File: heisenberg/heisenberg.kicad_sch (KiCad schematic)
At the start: 5 parts, among them J1 HLE-110-02-L-DV-BE-K-TR, J2 HLE-110-02-L-DV-BE-K-TR, J3 TSM-108-01-F-DV, J4 S16B-XH-A, U1 Teensy4.1

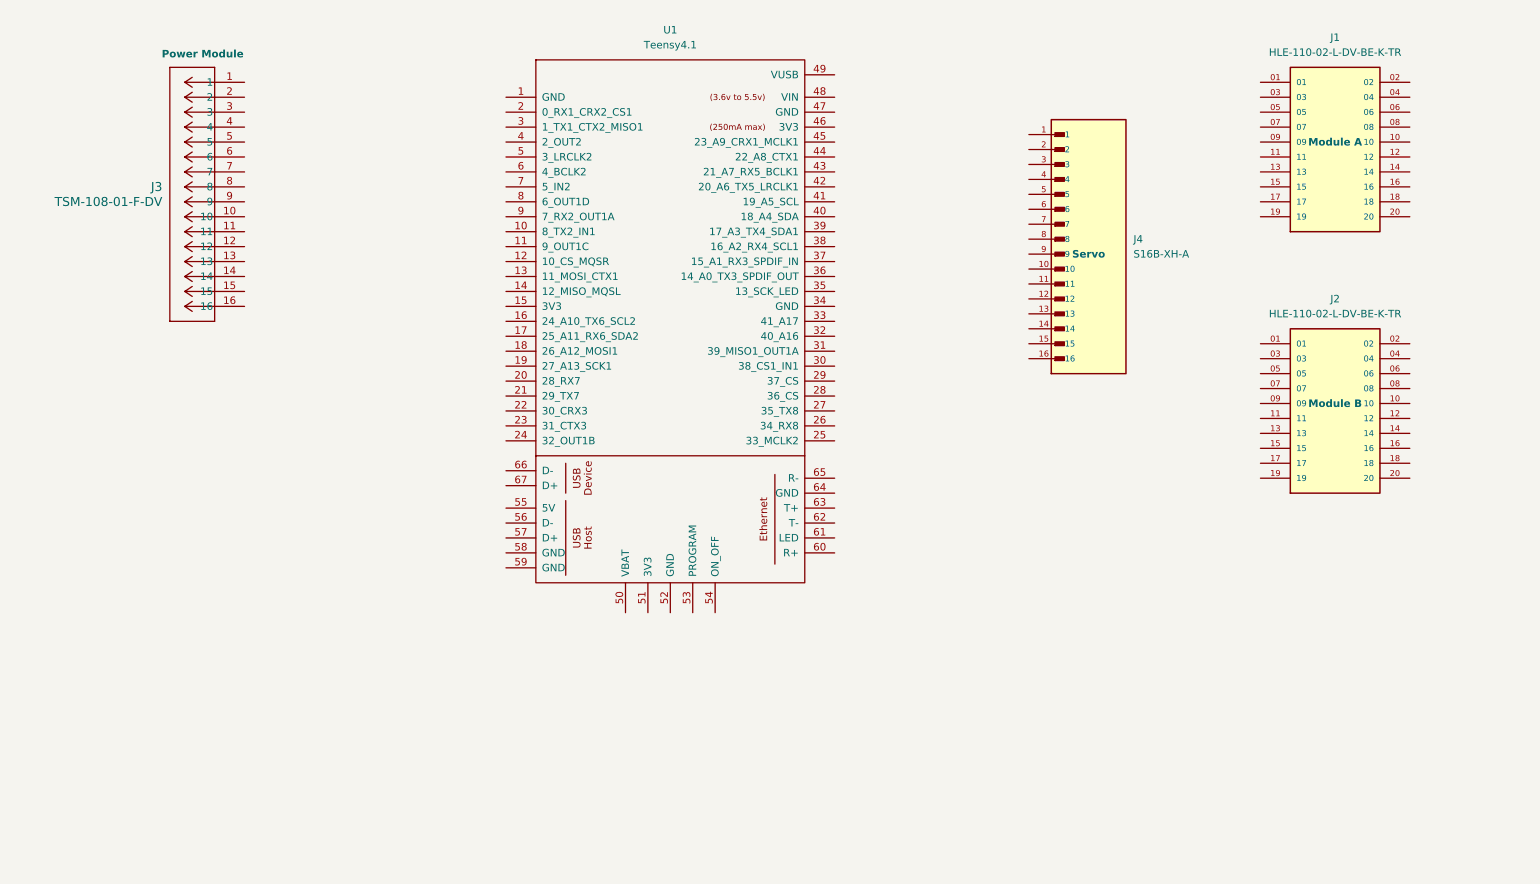
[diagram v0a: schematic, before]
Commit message: Main board MOD A&B pins & routing
V1 of  the initial module A & B routing so other people can have a starting point for their pin layout

dont mind the naming scheme i need to fix that
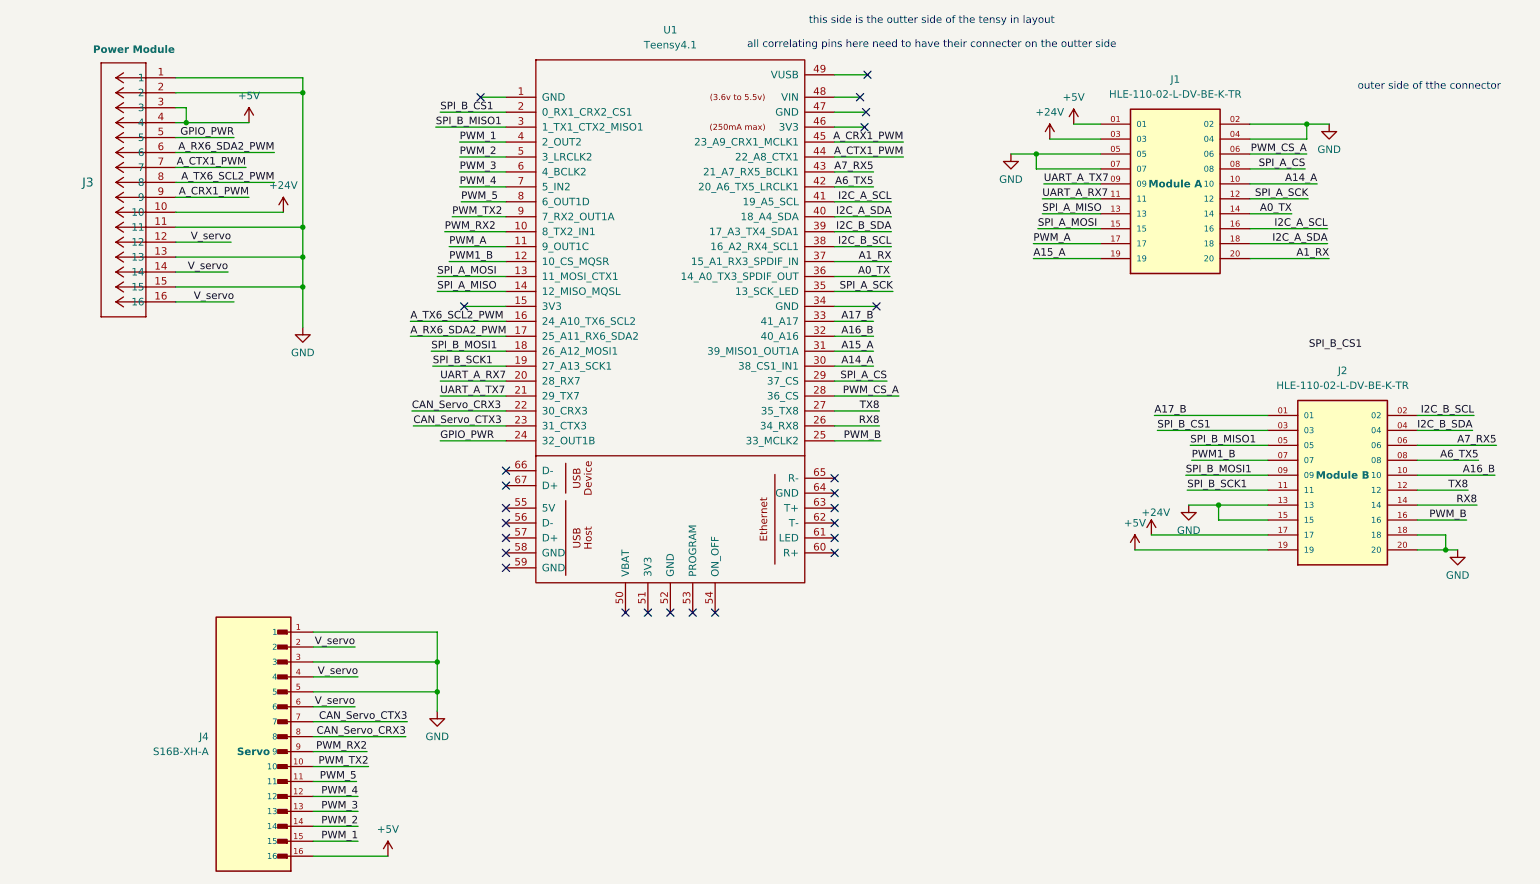
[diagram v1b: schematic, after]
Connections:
- net +5V: now reaches J1.01
- net +5V: now also J2.19, J3.3, J3.4, J4.16
- net GND: now reaches J1.02
- net GND: now also J1.04, J1.05, J1.07, J2.13, J2.15, J2.18, J2.20, J3.1, J3.11, J3.13, J3.15, J3.2, J4.1, J4.3, J4.5
- net +24V: now reaches J1.03
- net +24V: now also J2.17, J3.10
- net PWM_CS_A: now reaches J1.06
- net PWM_CS_A: now also U1.28 (36_CS)
- net SPI_A_CS: now reaches J1.08
- net SPI_A_CS: now also U1.29 (37_CS)
- net UART_A_TX7: now reaches J1.09
- net UART_A_TX7: now also U1.21 (29_TX7)
- net A14_A: now reaches J1.10
- net A14_A: now also U1.30 (38_CS1_IN1)
- net UART_A_RX7: now reaches J1.11
- net UART_A_RX7: now also U1.20 (28_RX7)
- net SPI_A_SCK: now reaches J1.12
- net SPI_A_SCK: now also U1.35 (13_SCK_LED)
- net SPI_A_MISO: now reaches J1.13
- net SPI_A_MISO: now also U1.14 (12_MISO_MQSL)
- net A0_TX: now reaches J1.14
- net A0_TX: now also U1.36 (14_A0_TX3_SPDIF_OUT)
- net SPI_A_MOSI: now reaches J1.15
- net SPI_A_MOSI: now also U1.13 (11_MOSI_CTX1)
- net I2C_A_SCL: now reaches J1.16
- net I2C_A_SCL: now also U1.41 (19_A5_SCL)
- net PWM_A: now reaches J1.17
- net PWM_A: now also U1.11 (9_OUT1C)
- net I2C_A_SDA: now reaches J1.18
- net I2C_A_SDA: now also U1.40 (18_A4_SDA)
- net A15_A: now reaches J1.19
- net A15_A: now also U1.31 (39_MISO1_OUT1A)
- net A1_RX: now reaches J1.20
- net A1_RX: now also U1.37 (15_A1_RX3_SPDIF_IN)
- net A17_B: now reaches J2.01
- net A17_B: now also U1.33 (41_A17)
- net I2C_B_SCL: now reaches J2.02
- net I2C_B_SCL: now also U1.38 (16_A2_RX4_SCL1)
- net SPI_B_CS1: now reaches J2.03
- net SPI_B_CS1: now also U1.2 (0_RX1_CRX2_CS1)
- net I2C_B_SDA: now reaches J2.04
- net I2C_B_SDA: now also U1.39 (17_A3_TX4_SDA1)
- net SPI_B_MISO1: now reaches J2.05
- net SPI_B_MISO1: now also U1.3 (1_TX1_CTX2_MISO1)
- net A7_RX5: now reaches J2.06
- net A7_RX5: now also U1.43 (21_A7_RX5_BCLK1)
- net PWM1_B: now reaches J2.07
- net PWM1_B: now also U1.12 (10_CS_MQSR)
- net A6_TX5: now reaches J2.08
- net A6_TX5: now also U1.42 (20_A6_TX5_LRCLK1)
- net SPI_B_MOSI1: now reaches J2.09
- net SPI_B_MOSI1: now also U1.18 (26_A12_MOSI1)
- net A16_B: now reaches J2.10
- net A16_B: now also U1.32 (40_A16)
- net SPI_B_SCK1: now reaches J2.11
- net SPI_B_SCK1: now also U1.19 (27_A13_SCK1)
- net TX8: now reaches J2.12
- net TX8: now also U1.27 (35_TX8)
- net RX8: now reaches J2.14
- net RX8: now also U1.26 (34_RX8)
- net PWM_B: now reaches J2.16
- net PWM_B: now also U1.25 (33_MCLK2)
- net V_servo: now reaches J3.12
- net V_servo: now also J3.14, J3.16, J4.2, J4.4, J4.6
- net GPIO_PWR: now reaches J3.5
- net GPIO_PWR: now also U1.24 (32_OUT1B)
- net A_RX6_SDA2_PWM: now reaches J3.6
- net A_RX6_SDA2_PWM: now also U1.17 (25_A11_RX6_SDA2)
- net A_CTX1_PWM: now reaches J3.7
- net A_CTX1_PWM: now also U1.44 (22_A8_CTX1)
- net A_TX6_SCL2_PWM: now reaches J3.8
- net A_TX6_SCL2_PWM: now also U1.16 (24_A10_TX6_SCL2)
- net A_CRX1_PWM: now reaches J3.9
- net A_CRX1_PWM: now also U1.45 (23_A9_CRX1_MCLK1)
- net PWM_TX2: now reaches J4.10
- net PWM_TX2: now also U1.9 (7_RX2_OUT1A)
- net PWM_5: now reaches J4.11
- net PWM_5: now also U1.8 (6_OUT1D)
- net PWM_4: now reaches J4.12
- net PWM_4: now also U1.7 (5_IN2)
- net PWM_3: now reaches J4.13
- net PWM_3: now also U1.6 (4_BCLK2)
- net PWM_2: now reaches J4.14
- net PWM_2: now also U1.5 (3_LRCLK2)
- net PWM_1: now reaches J4.15
- net PWM_1: now also U1.4 (2_OUT2)
- net CAN_Servo_CTX3: now reaches J4.7
- net CAN_Servo_CTX3: now also U1.23 (31_CTX3)
- net CAN_Servo_CRX3: now reaches J4.8
- net CAN_Servo_CRX3: now also U1.22 (30_CRX3)
- net PWM_RX2: now reaches J4.9
- net PWM_RX2: now also U1.10 (8_TX2_IN1)
- no-connect marks 0 -> 25
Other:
- note added: "outer side of tthe connector"
- note added: "this side is the outter side of the tensy in layout all correlating pins here need to have their connecter on the outter side"
- moved on the sheet: J1, J2, J3, J4
